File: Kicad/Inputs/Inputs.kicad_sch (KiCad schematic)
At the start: 8 parts, among them J1 5V, J4 Ground

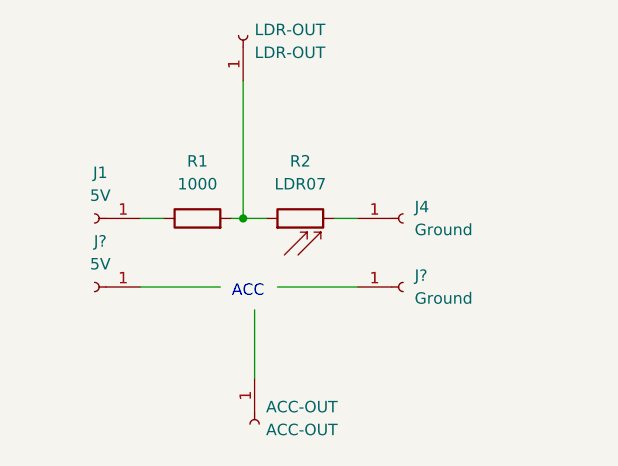
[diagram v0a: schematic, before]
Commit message: Update
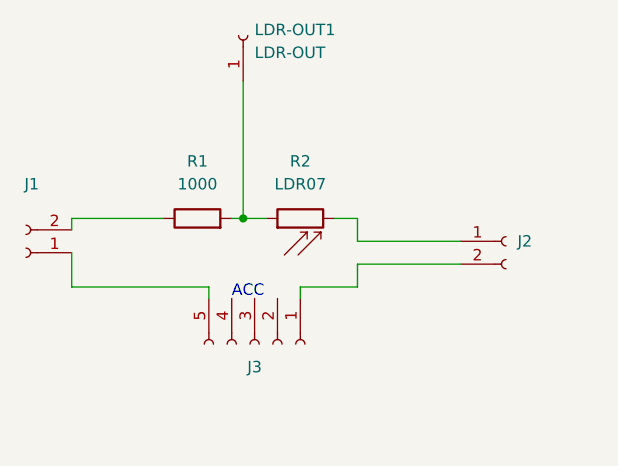
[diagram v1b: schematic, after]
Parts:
- removed ACC-OUT: ACC-OUT, Connector_PinHeader_1.00mm:PinHeader_1x01_P1.00mm_Vertical, symbol Connector:Conn_01x01_Female
- removed J1: 5V, symbol Connector:Conn_01x01_Female
- removed J4, J?: Ground, Connector_PinHeader_1.00mm:PinHeader_1x01_P1.00mm_Vertical, symbol Connector:Conn_01x01_Female
- removed J?: 5V, Connector_PinHeader_1.00mm:PinHeader_1x01_P1.00mm_Vertical, symbol Connector:Conn_01x01_Female
- added J1, J2: (no value), symbol Connector:Conn_01x02_Female
- added J3: (no value), symbol Connector:Conn_01x05_Female
- renumbered LDR-OUT to LDR-OUT1
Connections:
- net at R1.1: now also J1.2 (Pin_2)
- net at R2.2: now also J2.1 (Pin_1)
- new net: J1.1 (Pin_1), J3.5 (Pin_5)
- new net: J2.2 (Pin_2), J3.1 (Pin_1)
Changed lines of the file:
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@@
   (junction (at 135.89 93.98) (diameter 0) (color 0 0 0 0)
   )
+  (wire (pts (xy 116.84 101.6) (xy 132.08 101.6))
+    (stroke (width 0) (type default) (color 0 0 0 0))
+  )
+  (wire (pts (xy 148.59 101.6) (xy 142.24 101.6))
+    (stroke (width 0) (type default) (color 0 0 0 0))
+  )
   (wire (pts (xy 135.89 93.98) (xy 138.43 93.98))
+    (stroke (width 0) (type default) (color 0 0 0 0))
+  )
+  (wire (pts (xy 148.59 99.06) (xy 160.02 99.06))
+    (stroke (width 0) (type default) (color 0 0 0 0))
+  )
+  (wire (pts (xy 160.02 96.52) (xy 148.59 96.52))
+    (stroke (width 0) (type default) (color 0 0 0 0))
+  )
+  (wire (pts (xy 116.84 101.6) (xy 116.84 97.79))
+    (stroke (width 0) (type default) (color 0 0 0 0))
+  )
+  (wire (pts (xy 116.84 93.98) (xy 116.84 95.25))
+    (stroke (width 0) (type default) (color 0 0 0 0))
+  )
+  (wire (pts (xy 132.08 101.6) (xy 132.08 102.87))
     (stroke (width 0) (type default) (color 0 0 0 0))
   )
@@
     (stroke (width 0) (type default) (color 0 0 0 0))
   )
-  (wire (pts (xy 139.7 101.6) (xy 148.59 101.6))
+  (wire (pts (xy 142.24 101.6) (xy 142.24 102.87))
     (stroke (width 0) (type default) (color 0 0 0 0))
   )
-  (wire (pts (xy 137.16 104.14) (xy 137.16 111.76))
+  (wire (pts (xy 148.59 101.6) (xy 148.59 99.06))
     (stroke (width 0) (type default) (color 0 0 0 0))
   )
-  (wire (pts (xy 124.46 93.98) (xy 127 93.98))
+  (wire (pts (xy 116.84 93.98) (xy 127 93.98))
     (stroke (width 0) (type default) (color 0 0 0 0))
   )
@@
     (stroke (width 0) (type default) (color 0 0 0 0))
   )
-  (wire (pts (xy 124.46 101.6) (xy 133.35 101.6))
+  (wire (pts (xy 148.59 96.52) (xy 148.59 93.98))
     (stroke (width 0) (type default) (color 0 0 0 0))
   )
@@
     (effects (font (size 1.27 1.27)) (justify left bottom))
   )
-  (symbol (lib_id "Connector:Conn_01x01_Female") (at 137.16 116.84 270) (unit 1)
+  (symbol (lib_id "Connector:Conn_01x02_Female") (at 111.76 97.79 180) (unit 1)
     (in_bom yes) (on_board yes) (fields_autoplaced)
-    (property "Reference" "ACC-OUT" (id 0) (at 138.43 114.9349 90)
-      (effects (font (size 1.27 1.27)) (justify left))
-    )
-    (property "Value" "ACC-OUT" (id 1) (at 138.43 117.4749 90)
-      (effects (font (size 1.27 1.27)) (justify left))
-    )
-    (property "Footprint" "Connector_PinHeader_1.00mm:PinHeader_1x01_P1.00mm_Vertical" (id 2) (at 137.16 116.84 0)
+    (property "Reference" "J1" (id 0) (at 112.395 90.17 0))
+    (property "Value" "" (id 1) (at 112.395 92.71 0))
+    (property "Footprint" "" (id 2) (at 111.76 97.79 0)
       (effects (font (size 1.27 1.27)) hide)
     )
-    (property "Datasheet" "~" (id 3) (at 137.16 116.84 0)
+    (property "Datasheet" "~" (id 3) (at 111.76 97.79 0)
       (effects (font (size 1.27 1.27)) hide)
     )
     (pin "1")
+    (pin "2")
   )
-  (symbol (lib_id "Connector:Conn_01x01_Female") (at 119.38 93.98 180) (unit 1)
+  (symbol (lib_id "Connector:Conn_01x05_Female") (at 137.16 107.95 270) (unit 1)
     (in_bom yes) (on_board yes) (fields_autoplaced)
-    (property "Reference" "J1" (id 0) (at 120.015 88.9 0))
-    (property "Value" "5V" (id 1) (at 120.015 91.44 0))
-    (property "Footprint" "" (id 2) (at 119.38 93.98 0)
+    (property "Reference" "J3" (id 0) (at 137.16 110.49 90))
+    (property "Value" "" (id 1) (at 137.16 113.03 90))
+    (property "Footprint" "" (id 2) (at 137.16 107.95 0)
       (effects (font (size 1.27 1.27)) hide)
     )
-    (property "Datasheet" "~" (id 3) (at 119.38 93.98 0)
+    (property "Datasheet" "~" (id 3) (at 137.16 107.95 0)
       (effects (font (size 1.27 1.27)) hide)
     )
     (pin "1")
-  )
-  (symbol (lib_id "Connector:Conn_01x01_Female") (at 153.67 93.98 0) (unit 1)
-    (in_bom yes) (on_board yes) (fields_autoplaced)
-    (property "Reference" "J4" (id 0) (at 154.94 92.7099 0)
-      (effects (font (size 1.27 1.27)) (justify left))
-    )
-    (property "Value" "Ground" (id 1) (at 154.94 95.2499 0)
-      (effects (font (size 1.27 1.27)) (justify left))
-    )
-    (property "Footprint" "Connector_PinHeader_1.00mm:PinHeader_1x01_P1.00mm_Vertical" (id 2) (at 153.67 93.98 0)
-      (effects (font (size 1.27 1.27)) hide)
-    )
-    (property "Datasheet" "~" (id 3) (at 153.67 93.98 0)
-      (effects (font (size 1.27 1.27)) hide)
-    )
-    (pin "1")
+    (pin "2")
+    (pin "3")
+    (pin "4")
+    (pin "5")
   )
   (symbol (lib_id "Sensor_Optical:LDR07") (at 142.24 93.98 90) (unit 1)
@@
     (pin "2")
   )
-  (symbol (lib_id "Connector:Conn_01x01_Female") (at 153.67 101.6 0) (unit 1)
+  (symbol (lib_id "Connector:Conn_01x02_Female") (at 165.1 96.52 0) (unit 1)
     (in_bom yes) (on_board yes) (fields_autoplaced)
-    (property "Reference" "J?" (id 0) (at 154.94 100.3299 0)
+    (property "Reference" "J2" (id 0) (at 166.37 96.5199 0)
       (effects (font (size 1.27 1.27)) (justify left))
     )
-    (property "Value" "Ground" (id 1) (at 154.94 102.8699 0)
+    (property "Value" "" (id 1) (at 166.37 99.0599 0)
       (effects (font (size 1.27 1.27)) (justify left))
     )
-    (property "Footprint" "Connector_PinHeader_1.00mm:PinHeader_1x01_P1.00mm_Vertical" (id 2) (at 153.67 101.6 0)
+    (property "Footprint" "" (id 2) (at 165.1 96.52 0)
       (effects (font (size 1.27 1.27)) hide)
     )
-    (property "Datasheet" "~" (id 3) (at 153.67 101.6 0)
+    (property "Datasheet" "~" (id 3) (at 165.1 96.52 0)
       (effects (font (size 1.27 1.27)) hide)
     )
     (pin "1")
+    (pin "2")
   )
   (symbol (lib_id "Connector:Conn_01x01_Female") (at 135.89 73.66 90) (unit 1)
     (in_bom yes) (on_board yes) (fields_autoplaced)
-    (property "Reference" "LDR-OUT" (id 0) (at 137.16 73.0249 90)
+    (property "Reference" "LDR-OUT1" (id 0) (at 137.16 73.0249 90)
       (effects (font (size 1.27 1.27)) (justify right))
     )
@@
     )
     (property "Datasheet" "~" (id 3) (at 135.89 73.66 0)
-      (effects (font (size 1.27 1.27)) hide)
-    )
-    (pin "1")
-  )
-  (symbol (lib_id "Connector:Conn_01x01_Female") (at 119.38 101.6 180) (unit 1)
-    (in_bom yes) (on_board yes) (fields_autoplaced)
-    (property "Reference" "J?" (id 0) (at 120.015 96.52 0))
-    (property "Value" "5V" (id 1) (at 120.015 99.06 0))
-    (property "Footprint" "Connector_PinHeader_1.00mm:PinHeader_1x01_P1.00mm_Vertical" (id 2) (at 119.38 101.6 0)
-      (effects (font (size 1.27 1.27)) hide)
-    )
-    (property "Datasheet" "~" (id 3) (at 119.38 101.6 0)
       (effects (font (size 1.27 1.27)) hide)
     )
@@
   )
   (symbol_instances
-    (path "/4d31f32a-13e8-4329-ba1d-e492ed85914a"
-      (reference "ACC-OUT") (unit 1) (value "ACC-OUT") (footprint "Connector_PinHeader_1.00mm:PinHeader_1x01_P1.00mm_Vertical")
+    (path "/3745d030-b1db-42b3-88e5-5fb982cc9164"
+      (reference "J1") (unit 1) (value "5V") (footprint "Connector_PinHeader_1.00mm:PinHeader_1x02_P1.00mm_Vertical")
     )
-    (path "/7dcd56a3-27a3-4843-9832-1b7d54d34c80"
-      (reference "J1") (unit 1) (value "5V") (footprint "Connector_PinHeader_1.00mm:PinHeader_1x01_P1.00mm_Vertical")
+    (path "/a4525e50-456e-4d57-9ad8-84d9d1c29cd7"
+      (reference "J2") (unit 1) (value "GROUND") (footprint "Connector_PinHeader_1.00mm:PinHeader_1x02_P1.00mm_Vertical")
     )
-    (path "/96d98e65-7d79-4c49-bb2a-2933357e6bb4"
-      (reference "J4") (unit 1) (value "Ground") (footprint "Connector_PinHeader_1.00mm:PinHeader_1x01_P1.00mm_Vertical")
-    )
-    (path "/c9bde4f9-40be-4db2-8bb9-41c09ed25e46"
-      (reference "J?") (unit 1) (value "Ground") (footprint "Connector_PinHeader_1.00mm:PinHeader_1x01_P1.00mm_Vertical")
-    )
-    (path "/f68e5cfd-c99e-4b8f-9d7a-57b979a76fcc"
-      (reference "J?") (unit 1) (value "5V") (footprint "Connector_PinHeader_1.00mm:PinHeader_1x01_P1.00mm_Vertical")
+    (path "/40ac37d7-712c-4511-8d0a-ea04408e3716"
+      (reference "J3") (unit 1) (value "Conn_01x05_Female") (footprint "Connector_PinHeader_1.00mm:PinHeader_1x05_P1.00mm_Vertical")
     )
     (path "/e4a71a3b-a58d-43d4-98e3-aa823820b3c9"
-      (reference "LDR-OUT") (unit 1) (value "LDR-OUT") (footprint "Connector_PinHeader_1.00mm:PinHeader_1x01_P1.00mm_Vertical")
+      (reference "LDR-OUT1") (unit 1) (value "LDR-OUT") (footprint "Connector_PinHeader_1.00mm:PinHeader_1x01_P1.00mm_Vertical")
     )
     (path "/ff324643-a300-47c0-a55a-1a8f6c128714"

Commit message: Fix
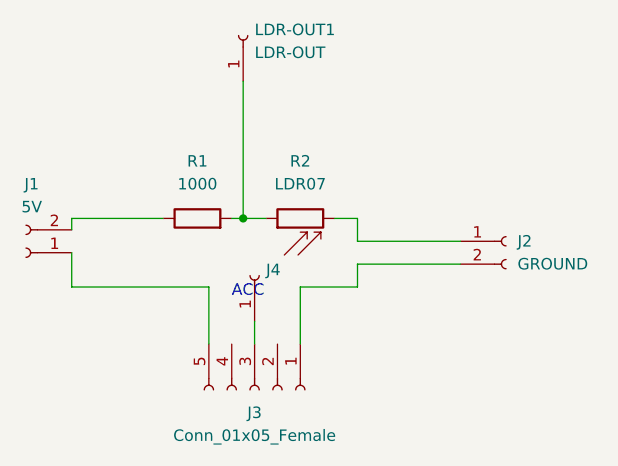
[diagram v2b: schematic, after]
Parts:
- added J4: (no value), symbol Connector:Conn_01x01_Female
- J1: value (none) -> 5V; footprint (none) -> Connector_PinHeader_1.00mm:PinHeader_1x02_P1.00mm_Vertical
- J2: value (none) -> GROUND; footprint (none) -> Connector_PinHeader_1.00mm:PinHeader_1x02_P1.00mm_Vertical
- J3: value (none) -> Conn_01x05_Female; footprint (none) -> Connector_PinHeader_1.00mm:PinHeader_1x05_P1.00mm_Vertical
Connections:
- net at J3.3 (Pin_3): now also J4.1 (Pin_1)
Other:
- moved on the sheet: J3
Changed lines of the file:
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@@
     (stroke (width 0) (type default) (color 0 0 0 0))
   )
-  (wire (pts (xy 132.08 101.6) (xy 132.08 102.87))
+  (wire (pts (xy 132.08 101.6) (xy 132.08 107.95))
     (stroke (width 0) (type default) (color 0 0 0 0))
   )
@@
     (stroke (width 0) (type default) (color 0 0 0 0))
   )
-  (wire (pts (xy 142.24 101.6) (xy 142.24 102.87))
+  (wire (pts (xy 137.16 105.41) (xy 137.16 107.95))
+    (stroke (width 0) (type default) (color 0 0 0 0))
+  )
+  (wire (pts (xy 142.24 101.6) (xy 142.24 107.95))
     (stroke (width 0) (type default) (color 0 0 0 0))
   )
@@
     (in_bom yes) (on_board yes) (fields_autoplaced)
     (property "Reference" "J1" (id 0) (at 112.395 90.17 0))
-    (property "Value" "" (id 1) (at 112.395 92.71 0))
-    (property "Footprint" "" (id 2) (at 111.76 97.79 0)
+    (property "Value" "5V" (id 1) (at 112.395 92.71 0))
+    (property "Footprint" "Connector_PinHeader_1.00mm:PinHeader_1x02_P1.00mm_Vertical" (id 2) (at 111.76 97.79 0)
       (effects (font (size 1.27 1.27)) hide)
     )
@@
     (pin "2")
   )
-  (symbol (lib_id "Connector:Conn_01x05_Female") (at 137.16 107.95 270) (unit 1)
+  (symbol (lib_id "Connector:Conn_01x05_Female") (at 137.16 113.03 270) (unit 1)
     (in_bom yes) (on_board yes) (fields_autoplaced)
-    (property "Reference" "J3" (id 0) (at 137.16 110.49 90))
-    (property "Value" "" (id 1) (at 137.16 113.03 90))
-    (property "Footprint" "" (id 2) (at 137.16 107.95 0)
+    (property "Reference" "J3" (id 0) (at 137.16 115.57 90))
+    (property "Value" "Conn_01x05_Female" (id 1) (at 137.16 118.11 90))
+    (property "Footprint" "Connector_PinHeader_1.00mm:PinHeader_1x05_P1.00mm_Vertical" (id 2) (at 137.16 113.03 0)
       (effects (font (size 1.27 1.27)) hide)
     )
-    (property "Datasheet" "~" (id 3) (at 137.16 107.95 0)
+    (property "Datasheet" "~" (id 3) (at 137.16 113.03 0)
       (effects (font (size 1.27 1.27)) hide)
     )
@@
     (pin "4")
     (pin "5")
+  )
+  (symbol (lib_id "Connector:Conn_01x01_Female") (at 137.16 100.33 90) (unit 1)
+    (in_bom yes) (on_board yes)
+    (property "Reference" "J4" (id 0) (at 138.43 99.6949 90)
+      (effects (font (size 1.27 1.27)) (justify right))
+    )
+    (property "Value" "" (id 1) (at 133.35 105.41 90)
+      (effects (font (size 1.27 1.27)) (justify right))
+    )
+    (property "Footprint" "" (id 2) (at 137.16 100.33 0)
+      (effects (font (size 1.27 1.27)) hide)
+    )
+    (property "Datasheet" "~" (id 3) (at 137.16 100.33 0)
+      (effects (font (size 1.27 1.27)) hide)
+    )
+    (pin "1")
   )
   (symbol (lib_id "Sensor_Optical:LDR07") (at 142.24 93.98 90) (unit 1)
@@
       (effects (font (size 1.27 1.27)) (justify left))
     )
-    (property "Value" "" (id 1) (at 166.37 99.0599 0)
+    (property "Value" "GROUND" (id 1) (at 166.37 99.0599 0)
       (effects (font (size 1.27 1.27)) (justify left))
     )
-    (property "Footprint" "" (id 2) (at 165.1 96.52 0)
+    (property "Footprint" "Connector_PinHeader_1.00mm:PinHeader_1x02_P1.00mm_Vertical" (id 2) (at 165.1 96.52 0)
       (effects (font (size 1.27 1.27)) hide)
     )
@@
       (reference "J3") (unit 1) (value "Conn_01x05_Female") (footprint "Connector_PinHeader_1.00mm:PinHeader_1x05_P1.00mm_Vertical")
     )
+    (path "/97973004-ab59-4480-8ec1-1121dd7cf977"
+      (reference "J4") (unit 1) (value "ACC OUT") (footprint "Connector_PinHeader_1.00mm:PinHeader_1x01_P1.00mm_Vertical")
+    )
     (path "/e4a71a3b-a58d-43d4-98e3-aa823820b3c9"
